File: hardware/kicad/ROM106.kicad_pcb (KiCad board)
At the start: 2 copper layers, 100 x 85 mm, 58 parts, among them J1 Screw_Terminal_01x03, J2 Screw_Terminal_01x03, J3 CAN, J4 Screw_Terminal_01x03, J5 Screw_Terminal_01x03, J6 Screw_Terminal_01x03, J7 Screw_Terminal_01x03, K1 PE014F05, K2 PE014F05, K3 PE014F05, K4 PE014F05, K5 PE014F05, K6 PE014F05, SW1 INSTANCE, SW2 BUS, SW3 PRG, U1 L293D, U2 MCP2551-I-P, U3 TMR_2411, U4 L293D, U5 L293D, U6 74HC595, U7 Teensy_3.2, U8 MAX6816

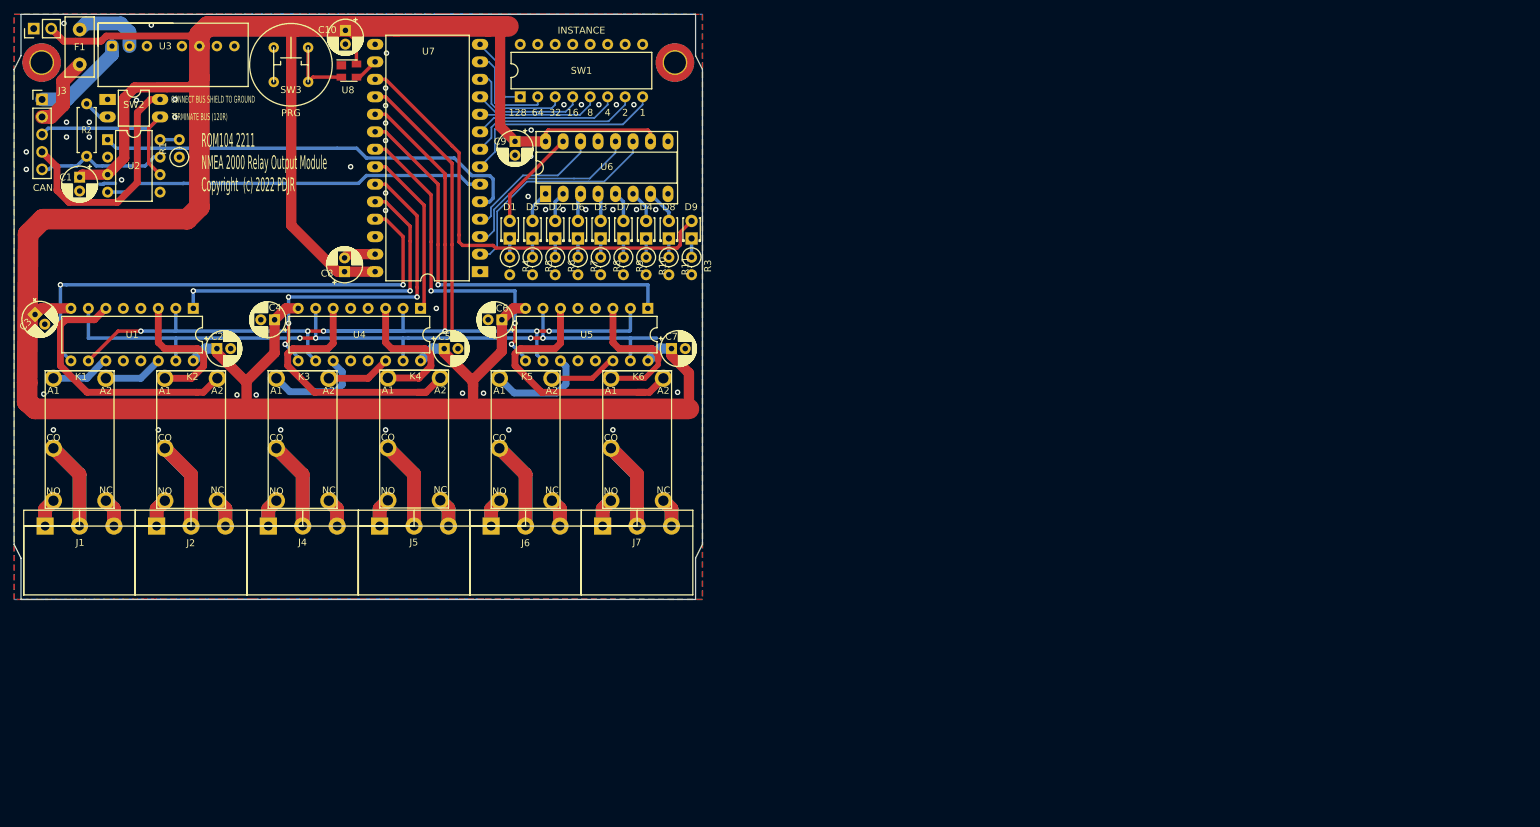
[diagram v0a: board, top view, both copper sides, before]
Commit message: Redraw PCB
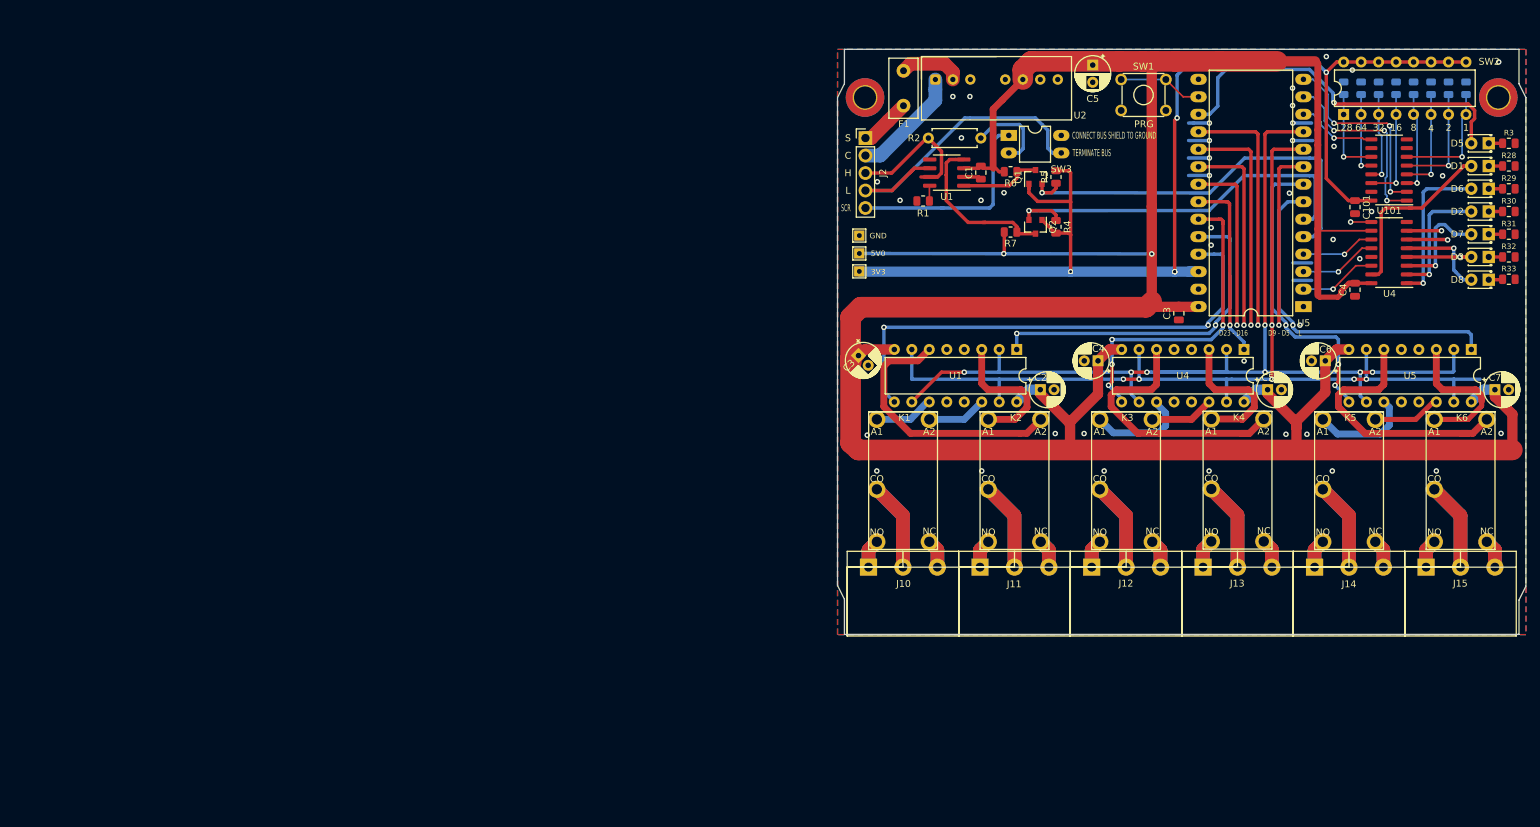
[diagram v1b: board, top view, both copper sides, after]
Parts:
- removed C10, C8, C9: 100nF, Capacitor_THT:CP_Radial_D5.0mm_P2.00mm
- removed D4, D9: LED, LED_THT:LED_D1.8mm_W3.3mm_H2.4mm
- removed J3: CAN, Connector_PinHeader_2.54mm:PinHeader_1x05_P2.54mm_Vertical
- removed R10, R11, R8, R9: 470R, Resistor_THT:R_Axial_DIN0207_L6.3mm_D2.5mm_P2.54mm_Vertical
- removed the REF** at (24.0, 27.0)
- removed the REF** at (116.0, 27.0)
- removed TEST: PinHeader_1x02_P2.54mm_Vertical, Connector_PinHeader_2.54mm:PinHeader_1x02_P2.54mm_Vertical
- removed U3: TMR_2411, PDJR_DC-DC_Converters:TMR_2411
- removed U6: 74HC595, Package_DIP:DIP-16_W7.62mm_Socket_LongPads
- removed U7: Teensy_3.2, Package_DIP:DIP-28_W15.24mm_LongPads
- removed U8: MAX6816, Package_TO_SOT_SMD:SOT-143
- added C101: 100nF, Capacitor_SMD:C_0805_2012Metric, F.Cu at (214.8, 48.0)
- added C3: 100nF, Capacitor_SMD:C_0805_2012Metric, F.Cu at (189.2, 63.4)
- added C4: 100nF, Capacitor_SMD:C_0805_2012Metric, F.Cu at (214.8, 60.0)
- added C5: 100nF, Capacitor_THT:CP_Radial_D5.0mm_P2.50mm, F.Cu at (176.7, 27.4)
- added J2: CAN, Connector_PinHeader_2.54mm:PinHeader_1x05_P2.54mm_Vertical, F.Cu at (143.7, 38.0)
- added Q1: BSS138, Package_TO_SOT_SMD:SOT-23, F.Cu at (168.4, 43.6)
- added Q2: BSS138, Package_TO_SOT_SMD:SOT-23, F.Cu at (168.4, 50.9)
- added R101: 4K7 0.125W, Resistor_SMD:R_0805_2012Metric, B.Cu at (230.9, 30.7)
- added R102: 4K7 0.125W, Resistor_SMD:R_0805_2012Metric, B.Cu at (228.4, 30.7)
- added R103: 4K7 0.125W, Resistor_SMD:R_0805_2012Metric, B.Cu at (225.8, 30.7)
- added R104: 4K7 0.125W, Resistor_SMD:R_0805_2012Metric, B.Cu at (223.3, 30.7)
- added R105: 4K7 0.125W, Resistor_SMD:R_0805_2012Metric, B.Cu at (220.8, 30.7)
- added R106: 4K7 0.125W, Resistor_SMD:R_0805_2012Metric, B.Cu at (218.2, 30.7)
- added R107: 4K7 0.125W, Resistor_SMD:R_0805_2012Metric, B.Cu at (215.7, 30.7)
- added R108: 4K7 0.125W, Resistor_SMD:R_0805_2012Metric, B.Cu at (213.1, 30.7)
- added R28: 560R, Resistor_SMD:R_0805_2012Metric, F.Cu at (237.1, 42.0)
- added R29: 560R, Resistor_SMD:R_0805_2012Metric, F.Cu at (237.1, 45.3)
- added R30: 560R, Resistor_SMD:R_0805_2012Metric, F.Cu at (237.1, 48.6)
- added R31: 560R, Resistor_SMD:R_0805_2012Metric, F.Cu at (237.1, 51.9)
- added R32: 560R, Resistor_SMD:R_0805_2012Metric, F.Cu at (237.1, 55.2)
- added R33: 560R, Resistor_SMD:R_0805_2012Metric, F.Cu at (237.1, 58.5)
- added REF**: TestPoint_THTPad_1.5x1.5mm_Drill0.7mm, TestPoint:TestPoint_THTPad_1.5x1.5mm_Drill0.7mm, F.Cu at (142.8, 52.1)
- added REF**: MountingHole_3.2mm_M3_DIN965_Pad_TopBottom, MountingHole:MountingHole_3.2mm_M3_DIN965_Pad_TopBottom, F.Cu at (143.6, 32.1)
- added REF**: MountingHole_3.2mm_M3_DIN965_Pad_TopBottom, MountingHole:MountingHole_3.2mm_M3_DIN965_Pad_TopBottom, F.Cu at (235.6, 32.1)
- added TEST 5V0: TestPoint_THTPad_1.5x1.5mm_Drill0.7mm, TestPoint:TestPoint_THTPad_1.5x1.5mm_Drill0.7mm, F.Cu at (142.8, 57.3)
- added TEST 5V0: TestPoint_THTPad_1.5x1.5mm_Drill0.7mm, TestPoint:TestPoint_THTPad_1.5x1.5mm_Drill0.7mm, F.Cu at (142.8, 54.7)
- added U1: MCP2551-I-P, Package_SO:SOIC-8_3.9x4.9mm_P1.27mm, F.Cu at (155.5, 43.0)
- added U101: 74HC165, Package_SO:SO-16_3.9x9.9mm_P1.27mm, F.Cu at (219.7, 42.6)
- added U4: 74HCT595, Package_SO:SO-16_3.9x9.9mm_P1.27mm, F.Cu at (219.7, 54.6)
- added U5: Teensy_4.0, Package_DIP:DIP-28_W15.24mm_LongPads, F.Cu at (207.3, 62.5)
- C1: footprint Capacitor_THT:CP_Radial_D5.0mm_P2.00mm -> Capacitor_SMD:C_0805_2012Metric
- R1: value 4K7 -> 4K7 0.125W; footprint Resistor_THT:R_Axial_DIN0207_L6.3mm_D2.5mm_P2.54mm_Vertical -> Resistor_SMD:R_0805_2012Metric
- R2: value 120R -> 120R 0.5W
- R3: value 470R -> 560R; footprint Resistor_THT:R_Axial_DIN0207_L6.3mm_D2.5mm_P2.54mm_Vertical -> Resistor_SMD:R_0805_2012Metric
- R4, R5, R6, R7: value 470R -> 10K 0.125W; footprint Resistor_THT:R_Axial_DIN0207_L6.3mm_D2.5mm_P2.54mm_Vertical -> Resistor_SMD:R_0805_2012Metric
- SW1: value INSTANCE -> PRG; footprint Package_DIP:DIP-16_W7.62mm -> Button_Switch_THT:SW_TH_Tactile_Omron_B3F-10xx
- SW2: value BUS -> INSTANCE; footprint Package_DIP:DIP-4_W7.62mm_LongPads -> Package_DIP:DIP-16_W7.62mm
- SW3: value PRG -> BUS; footprint PDJR-connectors:PCB_PUSH_BUTTON -> Package_DIP:DIP-4_W7.62mm_LongPads
- U2: value MCP2551-I-P -> TMR-2-2411; footprint Package_DIP:DIP-8_W7.62mm -> PDJR_DC-DC_Converters:TMR_2411
- moved SW2 179.6 mm to (213.1, 34.5), turned to 90 degrees
- moved D1 142.6 mm to (234.2, 42.0), turned to 180 degrees
- moved D5 139.6 mm to (234.2, 38.7), turned to 180 degrees
- moved D2 135.7 mm to (234.2, 48.6), turned to 180 degrees
- moved D6 132.5 mm to (234.2, 45.3), turned to 180 degrees
- moved C1 130.9 mm to (160.4, 43.0)
- moved D3 129.0 mm to (234.2, 55.2), turned to 180 degrees
- moved D7 125.7 mm to (234.2, 51.9), turned to 180 degrees
- moved R2 122.3 mm to (152.8, 38.0), turned to 0 degrees
- moved U2 120.6 mm to (153.8, 29.5)
- moved R3 119.9 mm to (237.1, 38.7), turned to 0 degrees
- moved F1 119.8 mm to (149.2, 33.3)
- moved C5 119.8 mm to (202.1, 74.5)
- moved J12 119.8 mm to (176.5, 100.3)
- moved J14 119.8 mm to (208.9, 100.3)
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- renumbered J1 to J10, J2 to J11, J4 to J12, J5 to J13, J6 to J14, J7 to J15
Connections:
- net /RST renamed /D9
- net /SET renamed /D8
- R2 pad 1: /CAN_H -> Net-(J2-Pad3)
- R2 pad 2: /TERM_A -> Net-(R2-Pad2)
- R3 pad 1: Net-(D9-Pad1) -> Net-(D5-Pad1)
- R4 pad 1: Net-(D1-Pad1) -> /CAN_RX
- R4 pad 2: GND -> +3V3
- R5 pad 1: Net-(D5-Pad1) -> /CAN_TX
- R5 pad 2: GND -> +3V3
- R6 pad 1: Net-(D2-Pad1) -> Net-(Q1-Pad3)
- R6 pad 2: GND -> +5V
- R7 pad 1: Net-(D6-Pad1) -> Net-(Q2-Pad3)
- R7 pad 2: GND -> +5V
- SW1 pad 1: /ADDR_0 -> /PRG
- SW1 pad 2: /ADDR_1 -> /PRG
- SW1 pad 3: /ADDR_2 -> GND
- SW1 pad 4: /ADDR_3 -> GND
- SW2 pad 1: GND -> Net-(R108-Pad1)
- SW2 pad 2: /TERM_A -> Net-(R107-Pad1)
- SW2 pad 3: /CAN_L -> Net-(R106-Pad1)
- SW2 pad 4: /CAN_SCR -> Net-(R105-Pad1)
- SW3 pad 1: GND -> Net-(J2-Pad5)
- SW3 pad 2: Net-(SW3-Pad2) -> Net-(R2-Pad2)
- U1 pad 1: /CH2_EN -> /D22
- U1 pad 9: /CH1_EN -> /D23
- U2 pad 1: /CAN_TX -> Net-(J2-Pad2)
- U2 pad 2: GND -> Net-(F1-Pad2)
- U2 pad 3: +5V -> (no net)
- U2 pad 5: Net-(U2-Pad5) -> (no net)
- U2 pad 6: /CAN_L -> +5V
- U2 pad 7: /CAN_H -> GND
- U2 pad 8: Net-(R1-Pad2) -> (no net)
- U4 pad 1: /CH4_EN -> /D20
- U4 pad 9: /CH3_EN -> /D21
- U5 pad 1: /CH6_EN -> /D5
- U5 pad 9: /CH5_EN -> /D6
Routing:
- net +3V3: track 0.00 -> 176.2 mm, vias 0 -> 5
- net /CH1_EN: track 73.6 -> 0.00 mm, vias 2 -> 0
- net /D23: track 0.00 -> 73.3 mm, vias 0 -> 2
- net /TRANSMIT_LED: track 66.4 -> 0.00 mm
- net /CH6_EN: track 60.8 -> 0.00 mm, vias 1 -> 0
- net /D5: track 0.00 -> 50.4 mm, vias 0 -> 1
- net /D22: track 0.00 -> 50.0 mm, vias 0 -> 2
- net /CH2_EN: track 50.0 -> 0.00 mm, vias 2 -> 0
- net /CH3_EN: track 48.7 -> 0.00 mm, vias 4 -> 0
- net Net-(D5-Pad2): track 4.73 -> 53.4 mm, vias 0 -> 1
- net /CH5_EN: track 48.2 -> 0.00 mm, vias 3 -> 0
- net Net-(J2-Pad4): track 0.00 -> 47.7 mm
- net /D21: track 0.00 -> 46.1 mm, vias 0 -> 4
- net /D6: track 0.00 -> 44.5 mm, vias 0 -> 3
- net /D16: track 0.00 -> 36.5 mm, vias 0 -> 1
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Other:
- outline, holes or cut-outs redrawn
- board text added: "3V3"
- board text added: "5V0"
- board text added: "C"
- board text added: "D23 - D16"
- board text added: "D9 - D5"
- board text added: "GND"
- board text added: "H"
- board text added: "L"
- board text added: "S"
- board text added: "SCR"
- board text added: "TERMINATE BUS"
- board text removed: "ROM104 2211 NMEA 2000 Relay Output Module Copyright (c) 2022 PDJR"
- board text removed: "TERMINATE BUS (120R)"

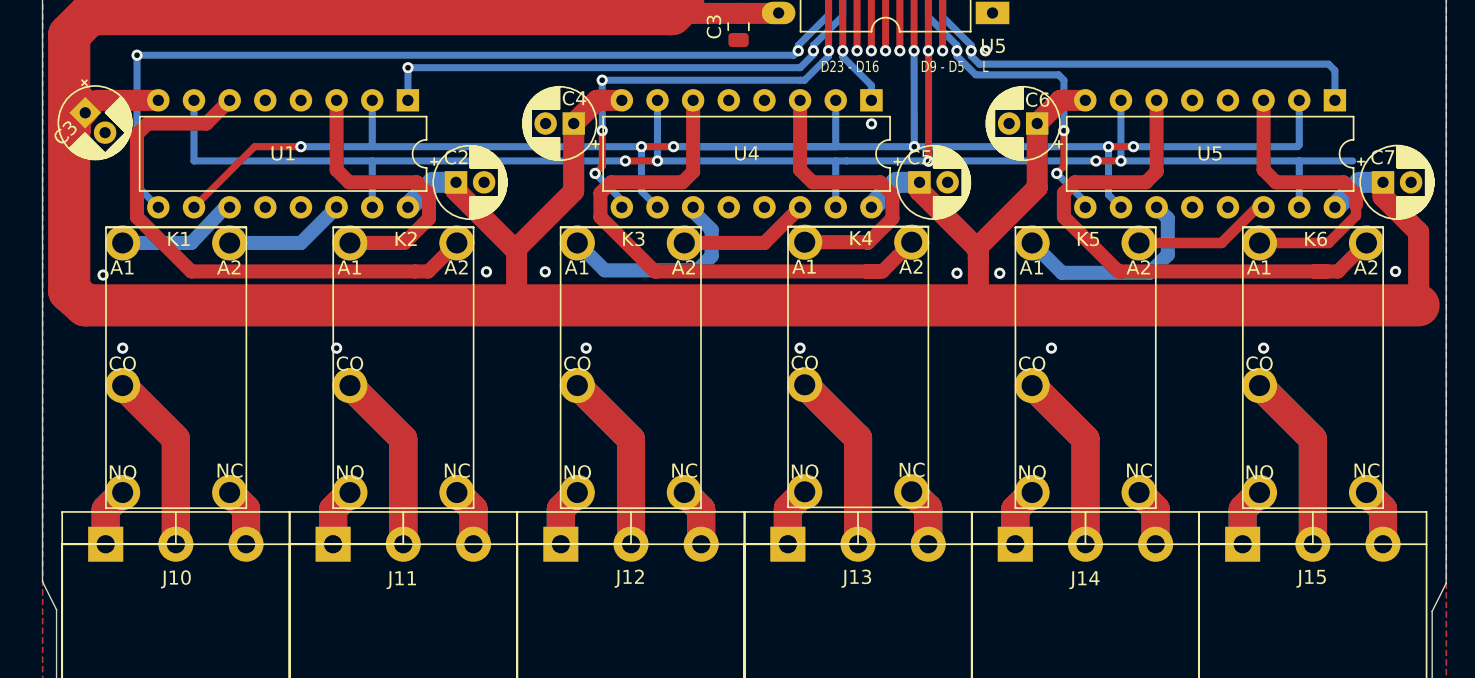
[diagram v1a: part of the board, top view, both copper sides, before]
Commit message: Tweak
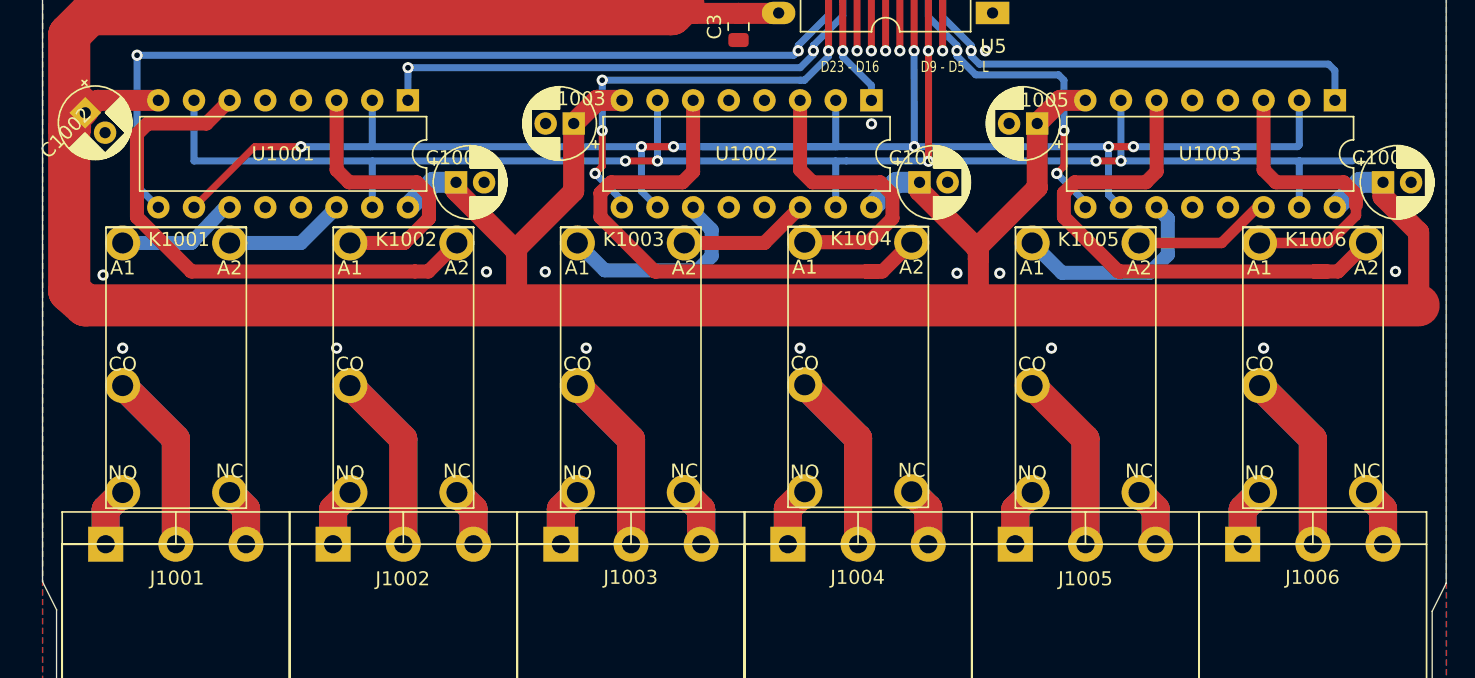
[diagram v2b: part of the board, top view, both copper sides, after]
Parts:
- renumbered C2 to C1001, C3 to C1002, C4 to C1003, C5 to C1004, C6 to C1005, C7 to C1006, J10 to J1001, J11 to J1002, J12 to J1003, J13 to J1004, J14 to J1005, J15 to J1006, K1 to K1001, K2 to K1002, K3 to K1003, K4 to K1004, K5 to K1005, K6 to K1006, U1 to U1001, U4 to U1002, U5 to U1003

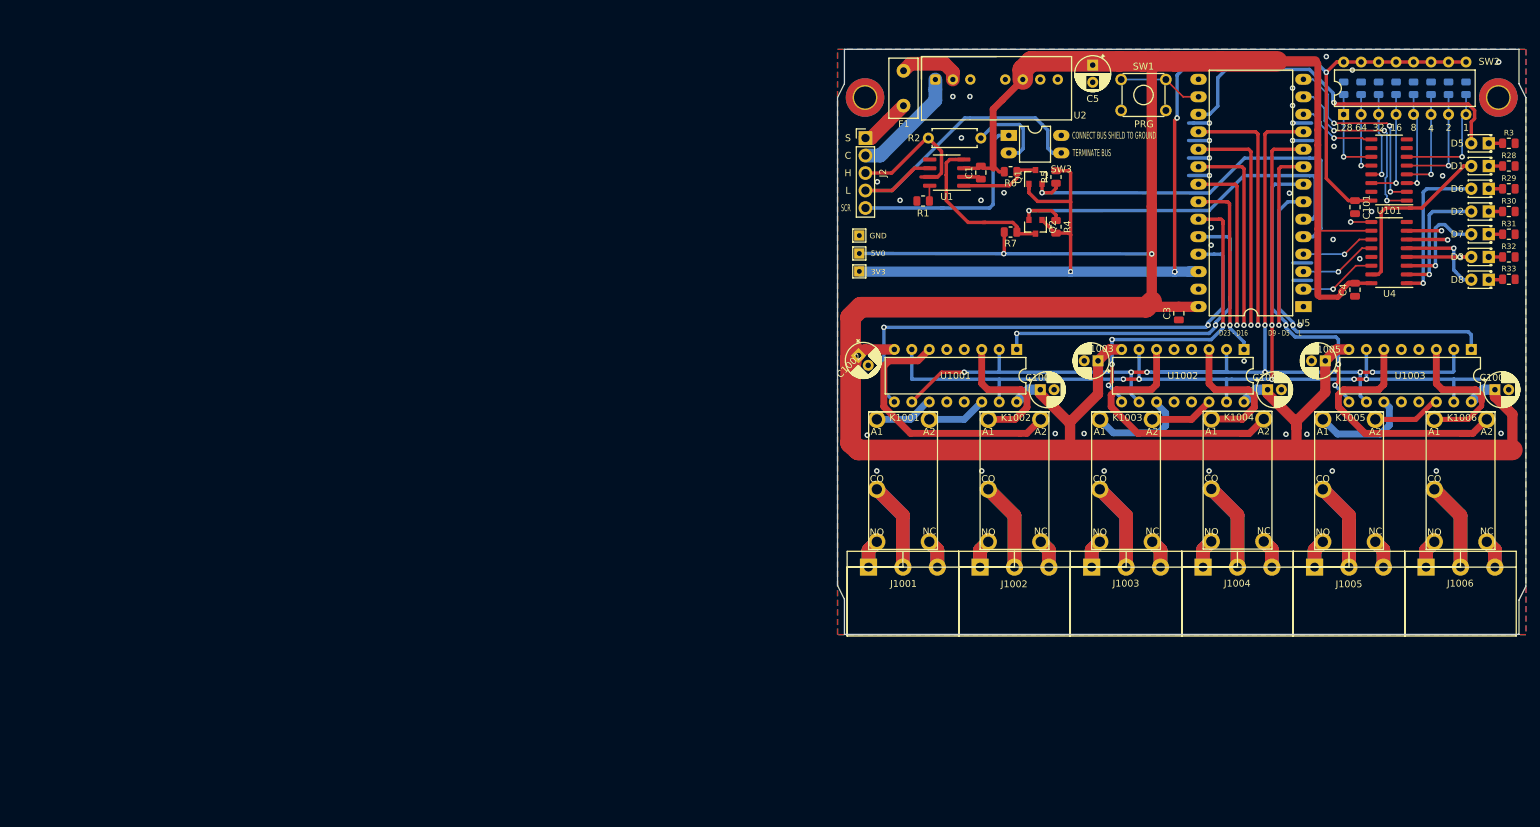
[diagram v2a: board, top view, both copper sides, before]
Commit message: Refactor
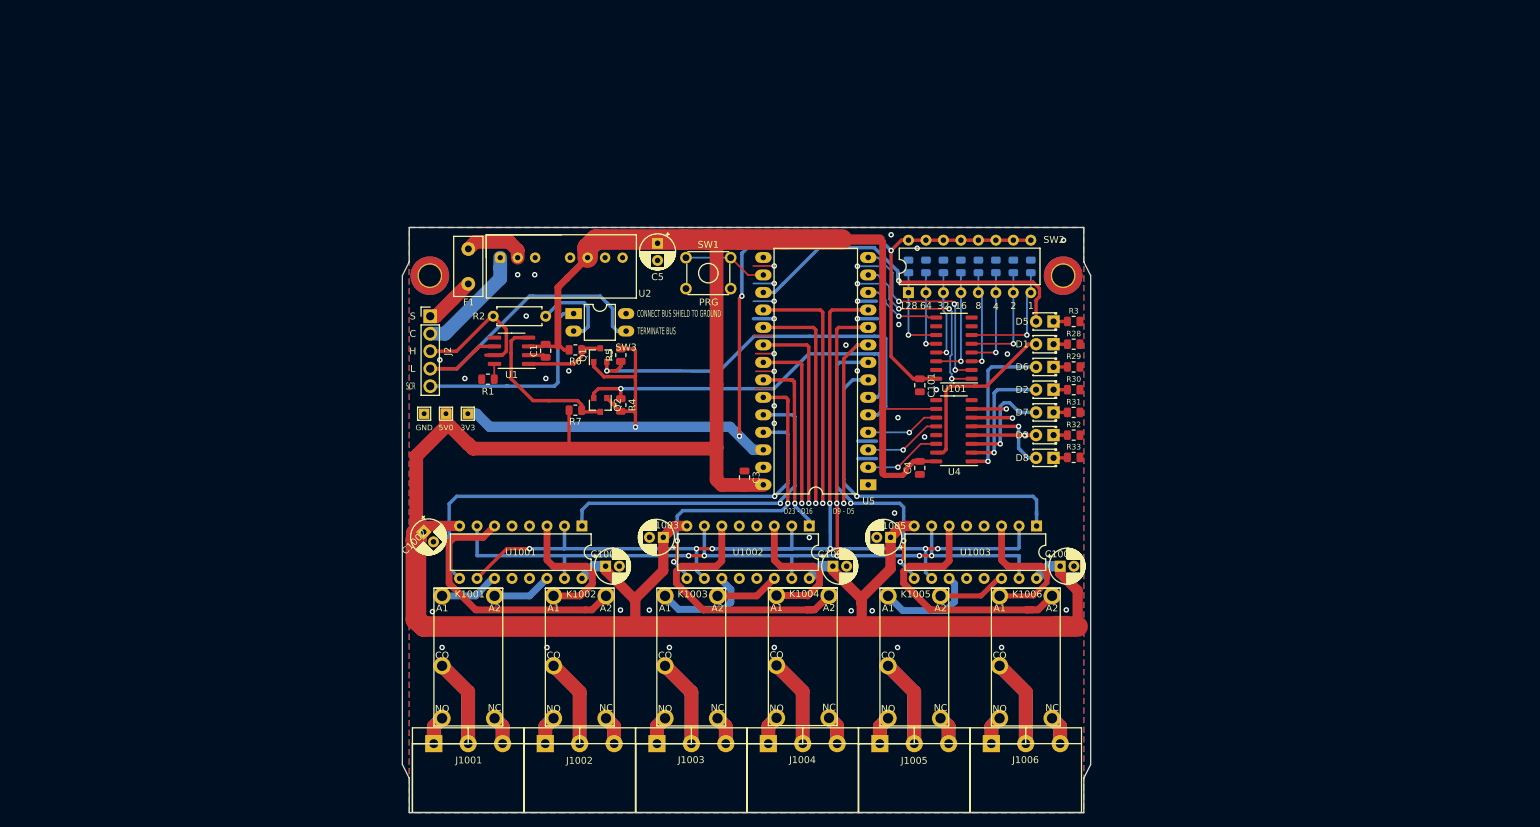
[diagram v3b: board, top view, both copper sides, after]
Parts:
- moved R103 68.3 mm to (162.6, 56.6)
- moved R106 68.3 mm to (155.0, 56.6)
- moved R107 68.3 mm to (152.5, 56.6)
- moved R28 68.3 mm to (173.9, 67.9)
- moved R29 68.3 mm to (173.9, 71.2)
- moved R3 68.3 mm to (173.9, 64.6)
- moved R30 68.3 mm to (173.9, 74.5)
- moved R31 68.3 mm to (173.9, 77.8)
- moved R32 68.3 mm to (173.9, 81.1)
- moved R33 68.3 mm to (173.9, 84.4)
- moved U101 68.3 mm to (156.5, 68.5)
- moved U4 68.3 mm to (156.5, 80.5)
- moved U5 68.3 mm to (144.1, 88.3)
- moved C1 68.3 mm to (97.2, 68.9)
- moved C5 68.3 mm to (113.5, 53.3)
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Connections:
- net /INSTANCE_CP renamed /PISO_CP
- net /INSTANCE_PL renamed /PISO_PL
- net /INSTANCE_Q7 renamed /PISO_Q7
- net /LED_CLOCK renamed /SIPO_CLOCK
- net /LED_DATA renamed /SIPO_DATA
- net /LED_LATCH renamed /SIPO_LATCH
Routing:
- net +5V: track 447.1 -> 418.2 mm, vias 2 -> 0
- net GND: track 26.3 -> 43.8 mm, vias 39 -> 43
- net +3V3: track 176.2 -> 164.9 mm, vias 5 -> 4
- net /CAN_RX: track 57.7 -> 53.8 mm
- net /D8: track 143.4 -> 139.5 mm
- net Net-(U3-Pad14): track 3.01 -> 0.00 mm, vias 1 -> 0
- net Net-(D5-Pad2): track 53.4 -> 51.0 mm
- net /D7: track 26.4 -> 25.4 mm
- net /D5: track 50.4 -> 51.1 mm
- net /D23: track 73.3 -> 72.7 mm, vias 2 -> 1
- net /D21: track 46.1 -> 45.7 mm, vias 4 -> 3
- net /D22: track 50.0 -> 49.7 mm, vias 2 -> 1
- net Net-(U3-Pad9): vias 1 -> 0
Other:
- outline, holes or cut-outs redrawn
- board text removed: "NMEA 2000 Temperature Sensor Module"
- board text removed: "PWR/TX"
- board text removed: "TSENSE"
